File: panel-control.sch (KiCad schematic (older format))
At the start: 63 parts, among them J1 POWER_CONN, J10 PWR_HAT, J11 BOOT, J2 PROG, J3 PWR, J4 40HAT, J5 HUB-75_A, J6 HUB-75_B, J7 USB_PWR, J8 FAN, J9 I2S, Q1 DMG2305UX, Q2 DMMT5401, Q3 DMG2305UX, Q4 S8050, SW1 POW, SW2 NRST, U1 TXS0108EPW, U2 TXS0108EPW, U3 TXS0108EPW, U4 HT7533-1, U7 STM32L031F6Px

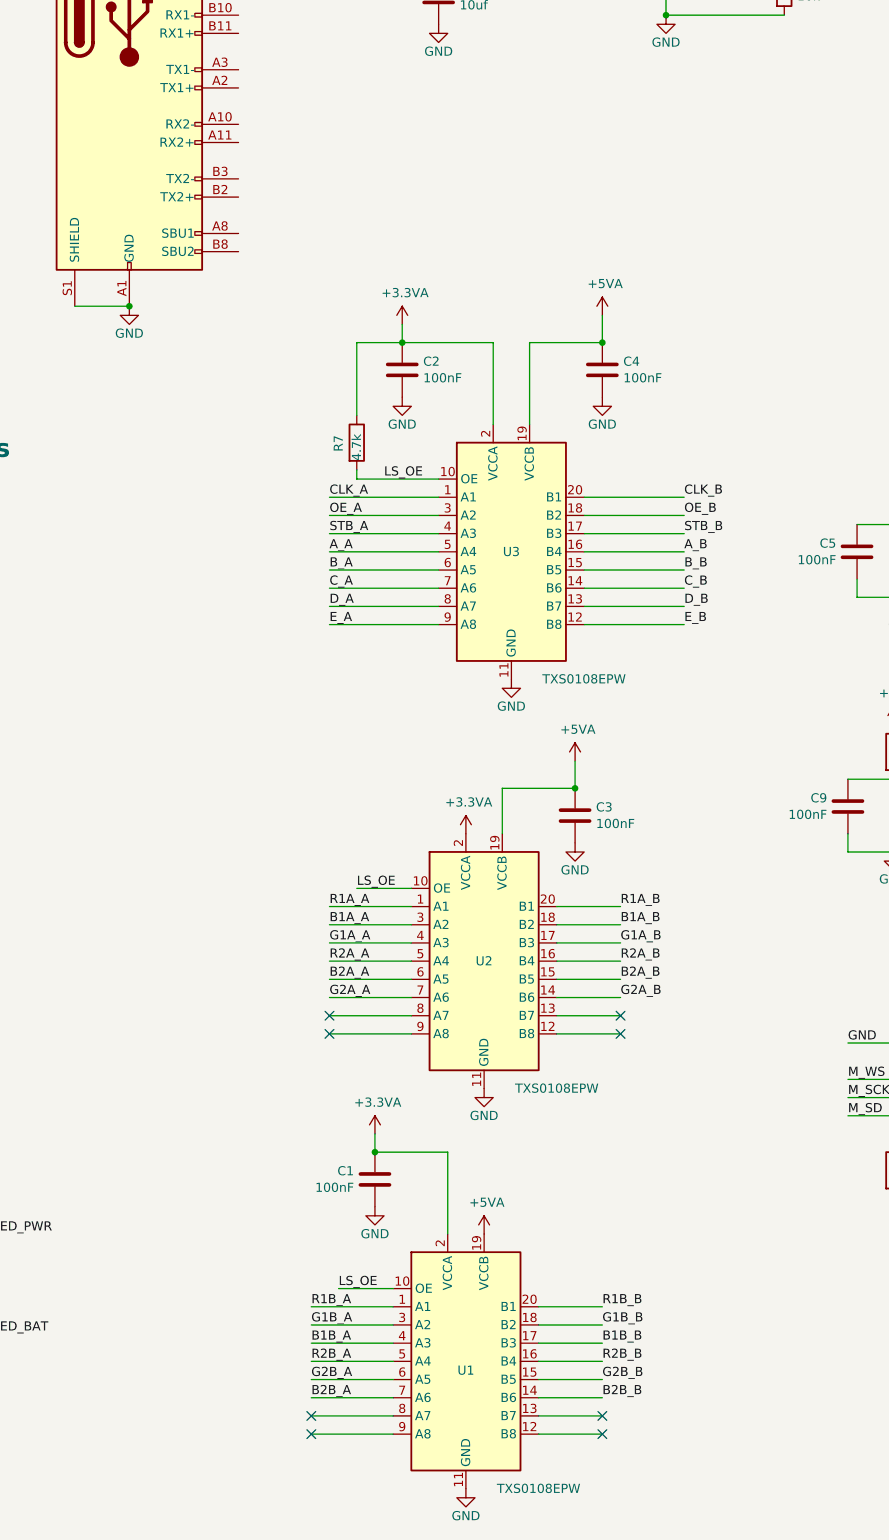
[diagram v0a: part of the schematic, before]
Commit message: finally submitted
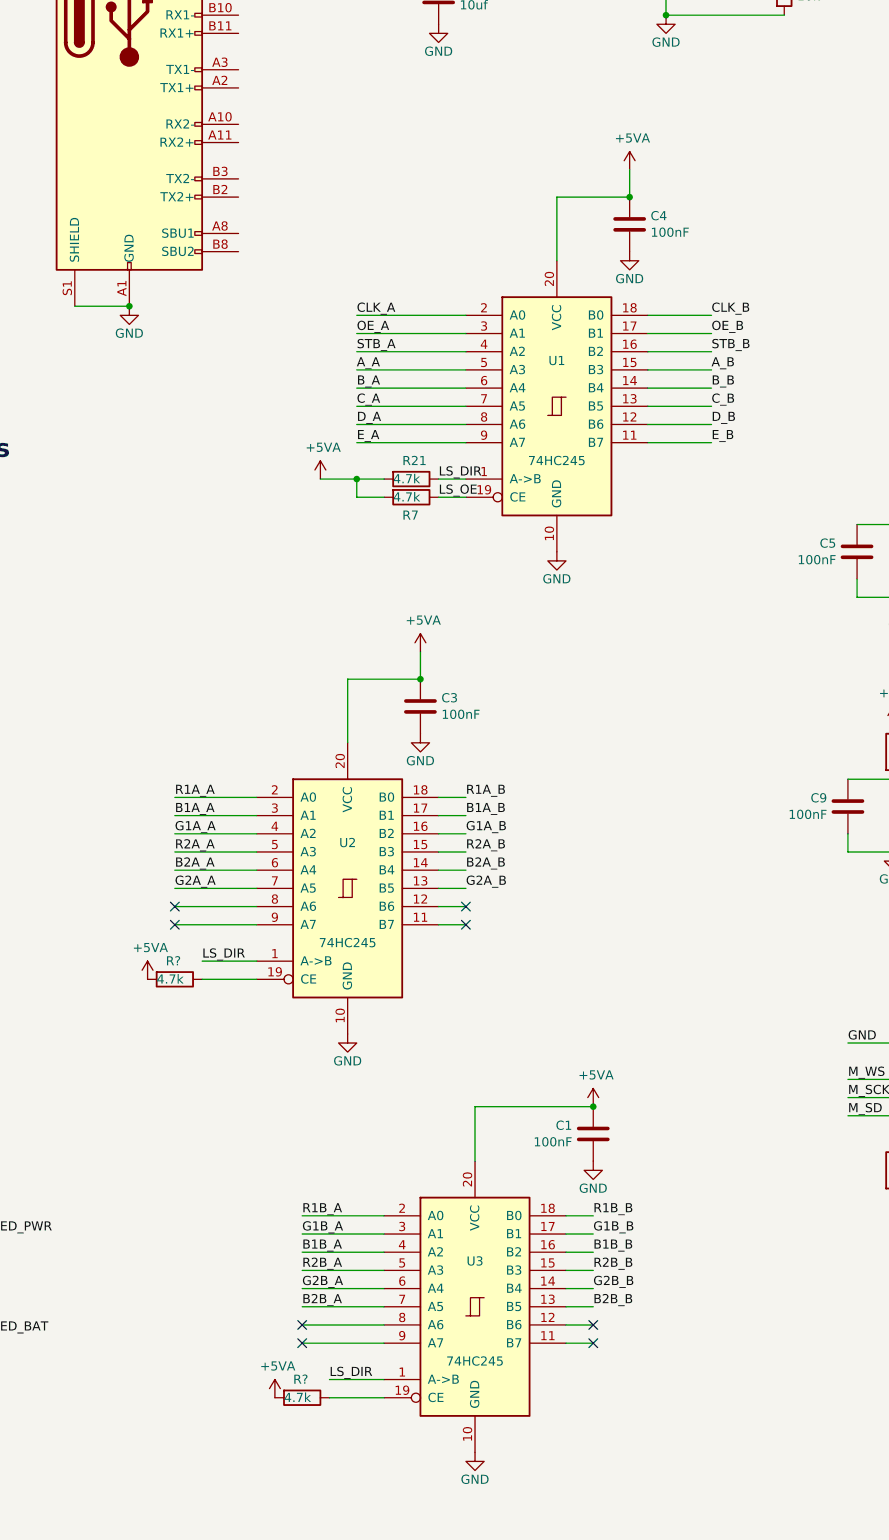
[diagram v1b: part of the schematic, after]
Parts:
- removed C2: 100nF, Capacitor_SMD:C_0603_1608Metric, symbol Device:C
- removed U1, U2, U3: TXS0108EPW, Package_SO:TSSOP-20_4.4x6.5mm_P0.65mm, symbol Logic_LevelTranslator:TXS0108EPW
- added R21, R? (x2): 4.7k, Resistor_SMD:R_0402_1005Metric, symbol Device:R
- added U1, U2, U3: 74HC245, Package_SO:SSOP-20_4.4x6.5mm_P0.65mm, symbol 74xx:74HC245
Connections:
- net +3.3VA: no longer C1.1, R7.1
- net +5VA: now also C1.1, R7.2, R21.2, R?.2, R?.2, U1.20 (VCC), U2.20 (VCC), U3.20 (VCC)
- net A_A: now also U1.5 (A3)
- net A_B: now also U1.15 (B3)
- net B1A_A: now also U2.3 (A1)
- net B1A_B: now also U2.17 (B1)
- net B1B_A: now also U3.4 (A2)
- net B1B_B: now also U3.16 (B2)
- net B2A_A: now also U2.6 (A4)
- net B2A_B: now also U2.14 (B4)
- net B2B_A: now also U3.7 (A5)
- net B2B_B: now also U3.13 (B5)
- net B_A: now also U1.6 (A4)
- net B_B: now also U1.14 (B4)
- net CLK_A: now also U1.2 (A0)
- net CLK_B: now also U1.18 (B0)
- net C_A: now also U1.7 (A5)
- net C_B: now also U1.13 (B5)
- net D_A: now also U1.8 (A6)
- net D_B: now also U1.12 (B6)
- net E_A: now also U1.9 (A7)
- net E_B: now also U1.11 (B7)
- net G1A_A: now also U2.4 (A2)
- net G1A_B: now also U2.16 (B2)
- net G1B_A: now also U3.3 (A1)
- net G1B_B: now also U3.17 (B1)
- net G2A_A: now also U2.7 (A5)
- net G2A_B: now also U2.13 (B5)
- net G2B_A: now also U3.6 (A4)
- net G2B_B: now also U3.14 (B4)
- net GND: now also U1.10 (GND), U2.10 (GND), U3.10 (GND)
- net LS_OE: now also R7.1, U1.19 (CE); no longer R7.2
- net OE_A: now also U1.3 (A1)
- net OE_B: now also U1.17 (B1)
- net R1A_A: now also U2.2 (A0)
- net R1A_B: now also U2.18 (B0)
- net R1B_A: now also U3.2 (A0)
- net R1B_B: now also U3.18 (B0)
- net R2A_A: now also U2.5 (A3)
- net R2A_B: now also U2.15 (B3)
- net R2B_A: now also U3.5 (A3)
- net R2B_B: now also U3.15 (B3)
- net STB_A: now also U1.4 (A2)
- net STB_B: now also U1.16 (B2)
- new net: R?.1, U2.19 (CE)
- new net: R?.1, U3.19 (CE)
- new net LS_DIR: R21.1, U1.1 (A->B), U2.1 (A->B), U3.1 (A->B)
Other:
- moved on the sheet: C1, C3, C4, R7
